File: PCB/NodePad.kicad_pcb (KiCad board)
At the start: 4 copper layers, 100 x 100 mm, 0 parts

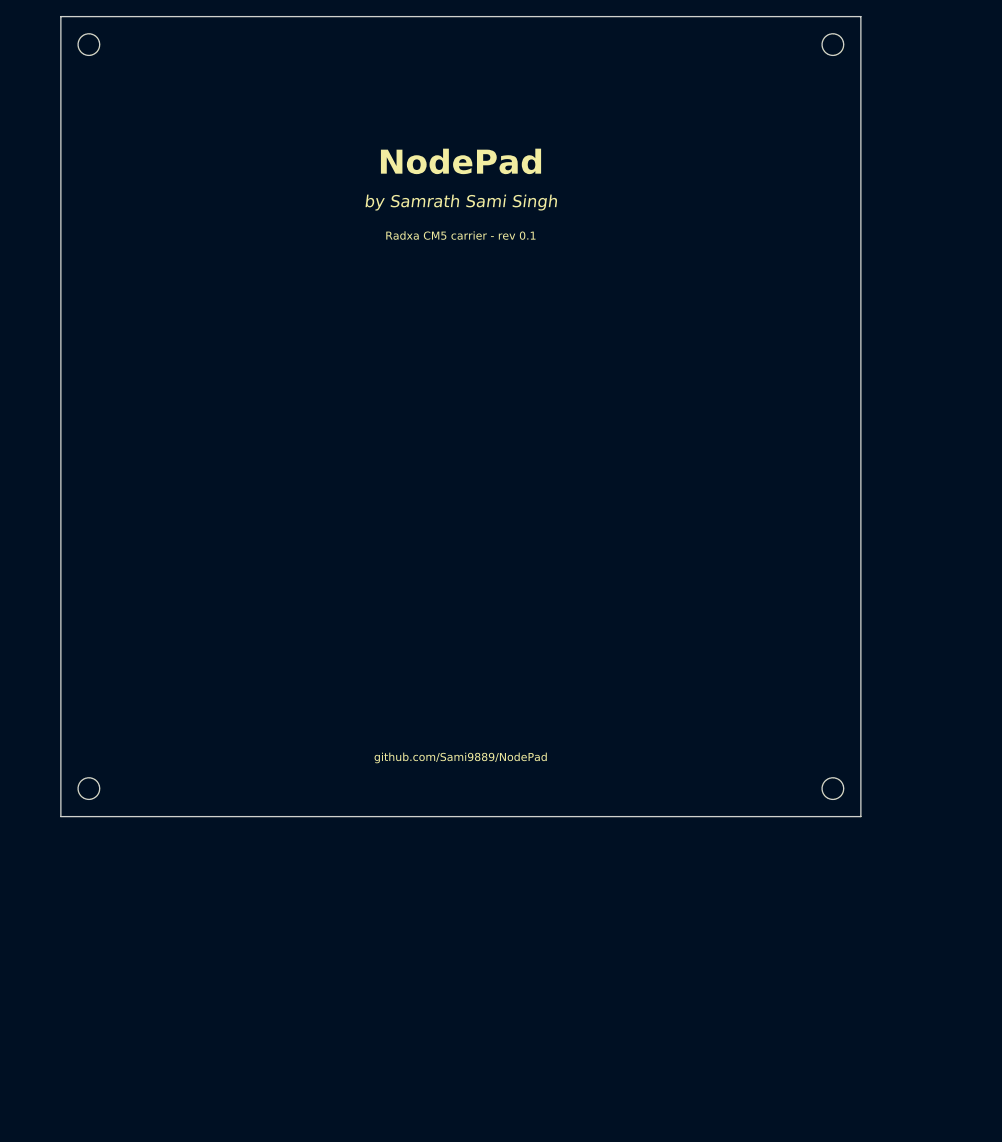
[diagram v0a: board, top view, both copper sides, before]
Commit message: Auto-generated changes
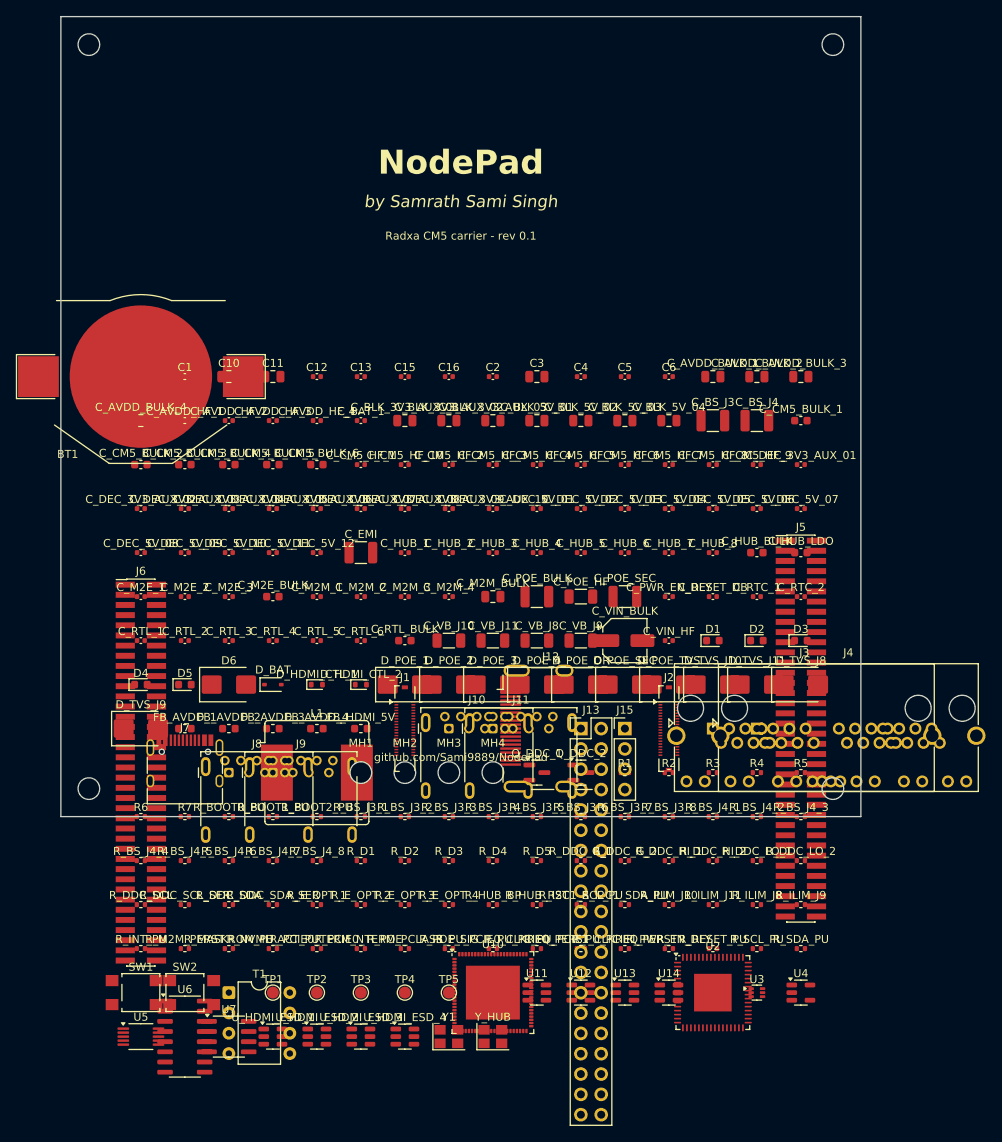
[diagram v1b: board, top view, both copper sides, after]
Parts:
- added BT1: CR2032, BatteryHolder_Keystone_3002_1x2032, F.Cu at (10.0, 45.0)
- added C1: 1uF, C_0402_1005Metric, F.Cu at (15.5, 45.0)
- added C10: 22uF/25V, C_0805_2012Metric, F.Cu at (21.0, 45.0)
- added C11: 22uF/25V, C_0805_2012Metric, F.Cu at (26.5, 45.0)
- added C12: 10uF/16V, C_0402_1005Metric, F.Cu at (32.0, 45.0)
- added C13: 100nF, C_0402_1005Metric, F.Cu at (37.5, 45.0)
- added C15: 1uF, C_0402_1005Metric, F.Cu at (43.0, 45.0)
- added C16: 1uF, C_0402_1005Metric, F.Cu at (48.5, 45.0)
- added C2: 1uF, C_0402_1005Metric, F.Cu at (54.0, 45.0)
- added C3: 22uF/25V, C_0805_2012Metric, F.Cu at (59.5, 45.0)
- added C4: 100nF, C_0402_1005Metric, F.Cu at (65.0, 45.0)
- added C5: 2.2nF, C_0402_1005Metric, F.Cu at (70.5, 45.0)
- added C6: 100pF, C_0402_1005Metric, F.Cu at (76.0, 45.0)
- added C_AVDD_BULK_1: 10uF, C_0805_2012Metric, F.Cu at (81.5, 45.0)
- added C_AVDD_BULK_2: 10uF, C_0805_2012Metric, F.Cu at (87.0, 45.0)
- added C_AVDD_BULK_3: 10uF, C_0805_2012Metric, F.Cu at (92.5, 45.0)
- added C_AVDD_BULK_4: 10uF, C_0805_2012Metric, F.Cu at (10.0, 50.5)
- added C_AVDD_HF_1: 100nF, C_0402_1005Metric, F.Cu at (15.5, 50.5)
- added C_AVDD_HF_2: 100nF, C_0402_1005Metric, F.Cu at (21.0, 50.5)
- added C_AVDD_HF_3: 100nF, C_0402_1005Metric, F.Cu at (26.5, 50.5)
- added C_AVDD_HF_4: 100nF, C_0402_1005Metric, F.Cu at (32.0, 50.5)
- added C_BAT_1: 100nF, C_0402_1005Metric, F.Cu at (37.5, 50.5)
- added C_BLK_3V3_AUX_01: 10uF, C_0805_2012Metric, F.Cu at (43.0, 50.5)
- added C_BLK_3V3_AUX_02: 10uF, C_0805_2012Metric, F.Cu at (48.5, 50.5)
- added C_BLK_3V3_AUX_03: 10uF, C_0805_2012Metric, F.Cu at (54.0, 50.5)
- added C_BLK_5V_01: 10uF, C_0805_2012Metric, F.Cu at (59.5, 50.5)
- added C_BLK_5V_02: 10uF, C_0805_2012Metric, F.Cu at (65.0, 50.5)
- added C_BLK_5V_03: 10uF, C_0805_2012Metric, F.Cu at (70.5, 50.5)
- added C_BLK_5V_04: 10uF, C_0805_2012Metric, F.Cu at (76.0, 50.5)
- added C_BS_J3: 1nF/2kV, C_1210_3225Metric, F.Cu at (81.5, 50.5)
- added C_BS_J4: 1nF/2kV, C_1210_3225Metric, F.Cu at (87.0, 50.5)
- added C_CM5_BULK_1: 10uF, C_0603_1608Metric, F.Cu at (92.5, 50.5)
- added C_CM5_BULK_2: 10uF, C_0603_1608Metric, F.Cu at (10.0, 56.0)
- added C_CM5_BULK_3: 10uF, C_0603_1608Metric, F.Cu at (15.5, 56.0)
- added C_CM5_BULK_4: 10uF, C_0603_1608Metric, F.Cu at (21.0, 56.0)
- added C_CM5_BULK_5: 10uF, C_0603_1608Metric, F.Cu at (26.5, 56.0)
- added C_CM5_BULK_6: 10uF, C_0603_1608Metric, F.Cu at (32.0, 56.0)
- added C_CM5_HF_1: 100nF, C_0402_1005Metric, F.Cu at (37.5, 56.0)
- added C_CM5_HF_10: 100nF, C_0402_1005Metric, F.Cu at (43.0, 56.0)
- added C_CM5_HF_2: 100nF, C_0402_1005Metric, F.Cu at (48.5, 56.0)
- added C_CM5_HF_3: 100nF, C_0402_1005Metric, F.Cu at (54.0, 56.0)
- added C_CM5_HF_4: 100nF, C_0402_1005Metric, F.Cu at (59.5, 56.0)
- added C_CM5_HF_5: 100nF, C_0402_1005Metric, F.Cu at (65.0, 56.0)
- added C_CM5_HF_6: 100nF, C_0402_1005Metric, F.Cu at (70.5, 56.0)
- added C_CM5_HF_7: 100nF, C_0402_1005Metric, F.Cu at (76.0, 56.0)
- added C_CM5_HF_8: 100nF, C_0402_1005Metric, F.Cu at (81.5, 56.0)
- added C_CM5_HF_9: 100nF, C_0402_1005Metric, F.Cu at (87.0, 56.0)
- added C_DEC_3V3_AUX_01: 100nF, C_0402_1005Metric, F.Cu at (92.5, 56.0)
- added C_DEC_3V3_AUX_02: 100nF, C_0402_1005Metric, F.Cu at (10.0, 61.5)
- added C_DEC_3V3_AUX_03: 100nF, C_0402_1005Metric, F.Cu at (15.5, 61.5)
- added C_DEC_3V3_AUX_04: 100nF, C_0402_1005Metric, F.Cu at (21.0, 61.5)
- added C_DEC_3V3_AUX_05: 100nF, C_0402_1005Metric, F.Cu at (26.5, 61.5)
- added C_DEC_3V3_AUX_06: 100nF, C_0402_1005Metric, F.Cu at (32.0, 61.5)
- added C_DEC_3V3_AUX_07: 100nF, C_0402_1005Metric, F.Cu at (37.5, 61.5)
- added C_DEC_3V3_AUX_08: 100nF, C_0402_1005Metric, F.Cu at (43.0, 61.5)
- added C_DEC_3V3_AUX_09: 100nF, C_0402_1005Metric, F.Cu at (48.5, 61.5)
- added C_DEC_3V3_AUX_10: 100nF, C_0402_1005Metric, F.Cu at (54.0, 61.5)
- added C_DEC_5V_01: 100nF, C_0402_1005Metric, F.Cu at (59.5, 61.5)
- added C_DEC_5V_02: 100nF, C_0402_1005Metric, F.Cu at (65.0, 61.5)
- added C_DEC_5V_03: 100nF, C_0402_1005Metric, F.Cu at (70.5, 61.5)
- added C_DEC_5V_04: 100nF, C_0402_1005Metric, F.Cu at (76.0, 61.5)
- added C_DEC_5V_05: 100nF, C_0402_1005Metric, F.Cu at (81.5, 61.5)
- added C_DEC_5V_06: 100nF, C_0402_1005Metric, F.Cu at (87.0, 61.5)
- added C_DEC_5V_07: 100nF, C_0402_1005Metric, F.Cu at (92.5, 61.5)
- added C_DEC_5V_08: 100nF, C_0402_1005Metric, F.Cu at (10.0, 67.0)
- added C_DEC_5V_09: 100nF, C_0402_1005Metric, F.Cu at (15.5, 67.0)
- added C_DEC_5V_10: 100nF, C_0402_1005Metric, F.Cu at (21.0, 67.0)
- added C_DEC_5V_11: 100nF, C_0402_1005Metric, F.Cu at (26.5, 67.0)
- added C_DEC_5V_12: 100nF, C_0402_1005Metric, F.Cu at (32.0, 67.0)
- added C_EMI: 1nF/2kV, C_1210_3225Metric, F.Cu at (37.5, 67.0)
- added C_HUB_1: 100nF, C_0402_1005Metric, F.Cu at (43.0, 67.0)
- added C_HUB_2: 100nF, C_0402_1005Metric, F.Cu at (48.5, 67.0)
- added C_HUB_3: 100nF, C_0402_1005Metric, F.Cu at (54.0, 67.0)
- added C_HUB_4: 100nF, C_0402_1005Metric, F.Cu at (59.5, 67.0)
- added C_HUB_5: 100nF, C_0402_1005Metric, F.Cu at (65.0, 67.0)
- added C_HUB_6: 100nF, C_0402_1005Metric, F.Cu at (70.5, 67.0)
- added C_HUB_7: 100nF, C_0402_1005Metric, F.Cu at (76.0, 67.0)
- added C_HUB_8: 100nF, C_0402_1005Metric, F.Cu at (81.5, 67.0)
- added C_HUB_BULK: 10uF, C_0603_1608Metric, F.Cu at (87.0, 67.0)
- added C_HUB_LDO: 4.7uF, C_0603_1608Metric, F.Cu at (92.5, 67.0)
- added C_M2E_1: 100nF, C_0402_1005Metric, F.Cu at (10.0, 72.5)
- added C_M2E_2: 100nF, C_0402_1005Metric, F.Cu at (15.5, 72.5)
- added C_M2E_3: 100nF, C_0402_1005Metric, F.Cu at (21.0, 72.5)
- added C_M2E_BULK: 10uF, C_0603_1608Metric, F.Cu at (26.5, 72.5)
- added C_M2M_1: 100nF, C_0402_1005Metric, F.Cu at (32.0, 72.5)
- added C_M2M_2: 100nF, C_0402_1005Metric, F.Cu at (37.5, 72.5)
- added C_M2M_3: 100nF, C_0402_1005Metric, F.Cu at (43.0, 72.5)
- added C_M2M_4: 100nF, C_0402_1005Metric, F.Cu at (48.5, 72.5)
- added C_M2M_BULK: 22uF/6.3V, C_0805_2012Metric, F.Cu at (54.0, 72.5)
- added C_POE_BULK: 22uF/100V DNP, C_1210_3225Metric, F.Cu at (59.5, 72.5)
- added C_POE_HF: 100nF/100V DNP, C_1206_3216Metric, F.Cu at (65.0, 72.5)
- added C_POE_SEC: 47uF/25V DNP, C_1210_3225Metric, F.Cu at (70.5, 72.5)
- added C_PWR_EN_DLY: 470nF, C_0402_1005Metric, F.Cu at (76.0, 72.5)
- added C_RESET_DB: 100nF, C_0402_1005Metric, F.Cu at (81.5, 72.5)
- added C_RTC_1: 100nF, C_0402_1005Metric, F.Cu at (87.0, 72.5)
- added C_RTC_2: 1uF, C_0402_1005Metric, F.Cu at (92.5, 72.5)
- added C_RTL_1: 100nF, C_0402_1005Metric, F.Cu at (10.0, 78.0)
- added C_RTL_2: 100nF, C_0402_1005Metric, F.Cu at (15.5, 78.0)
- added C_RTL_3: 100nF, C_0402_1005Metric, F.Cu at (21.0, 78.0)
- added C_RTL_4: 100nF, C_0402_1005Metric, F.Cu at (26.5, 78.0)
- added C_RTL_5: 100nF, C_0402_1005Metric, F.Cu at (32.0, 78.0)
- added C_RTL_6: 100nF, C_0402_1005Metric, F.Cu at (37.5, 78.0)
- added C_RTL_BULK: 10uF, C_0603_1608Metric, F.Cu at (43.0, 78.0)
- added C_VB_J10: 150uF/6.3V, C_1206_3216Metric, F.Cu at (48.5, 78.0)
- added C_VB_J11: 150uF/6.3V, C_1206_3216Metric, F.Cu at (54.0, 78.0)
- added C_VB_J8: 150uF/6.3V, C_1206_3216Metric, F.Cu at (59.5, 78.0)
- added C_VB_J9: 150uF/6.3V, C_1206_3216Metric, F.Cu at (65.0, 78.0)
- added C_VIN_BULK: 47uF/25V, CP_Elec_5x5.4, F.Cu at (70.5, 78.0)
- added C_VIN_HF: 100nF, C_0402_1005Metric, F.Cu at (76.0, 78.0)
- added D1: Green, LED_0603_1608Metric, F.Cu at (81.5, 78.0)
- added D2: Blue, LED_0603_1608Metric, F.Cu at (87.0, 78.0)
- added D3: Yellow, LED_0603_1608Metric, F.Cu at (92.5, 78.0)
- added D4: Yellow, LED_0603_1608Metric, F.Cu at (10.0, 83.5)
- added D5: Red, LED_0603_1608Metric, F.Cu at (15.5, 83.5)
- added D6: SMBJ12A, D_SMB, F.Cu at (21.0, 83.5)
- added D_BAT: BAT54, D_SOD-323, F.Cu at (26.5, 83.5)
- added D_HDMI_CTL_1: ESD5Z5.0, D_SOD-523, F.Cu at (32.0, 83.5)
- added D_HDMI_CTL_2: ESD5Z5.0, D_SOD-523, F.Cu at (37.5, 83.5)
- added D_POE_1: HD01-T DNP, D_SMB, F.Cu at (43.0, 83.5)
- added D_POE_2: HD01-T DNP, D_SMB, F.Cu at (48.5, 83.5)
- added D_POE_3: HD01-T DNP, D_SMB, F.Cu at (54.0, 83.5)
- added D_POE_4: HD01-T DNP, D_SMB, F.Cu at (59.5, 83.5)
- added D_POE_OR: SS36 DNP, D_SMB, F.Cu at (65.0, 83.5)
- added D_POE_SEC: SS36 DNP, D_SMB, F.Cu at (70.5, 83.5)
- added D_POE_TVS: SMBJ58A DNP, D_SMB, F.Cu at (76.0, 83.5)
- added D_TVS_J10: SMBJ5.0A, D_SMB, F.Cu at (81.5, 83.5)
- added D_TVS_J11: SMBJ5.0A, D_SMB, F.Cu at (87.0, 83.5)
- added D_TVS_J8: SMBJ5.0A, D_SMB, F.Cu at (92.5, 83.5)
- added D_TVS_J9: SMBJ5.0A, D_SMB, F.Cu at (10.0, 89.0)
- added FB_AVDD_1: 600R@100MHz, L_0603_1608Metric, F.Cu at (15.5, 89.0)
- added FB_AVDD_2: 600R@100MHz, L_0603_1608Metric, F.Cu at (21.0, 89.0)
- added FB_AVDD_3: 600R@100MHz, L_0603_1608Metric, F.Cu at (26.5, 89.0)
- added FB_AVDD_4: 600R@100MHz, L_0603_1608Metric, F.Cu at (32.0, 89.0)
- added FB_HDMI_5V: 600R@100MHz, L_0603_1608Metric, F.Cu at (37.5, 89.0)
- added J1: CM5-J1, Hirose_BM24_BM24-40DS-2-0.35V_2x20_P0.35mm_PowerPin2_Vertical, F.Cu at (43.0, 89.0)
- added J10: USB3-A, USB3_A_Molex_48393-001, F.Cu at (48.5, 89.0)
- added J11: USB3-A, USB3_A_Molex_48393-001, F.Cu at (54.0, 89.0)
- added J12: HDMI, HDMI_A_Molex_208658-1001_Horizontal, F.Cu at (59.5, 89.0)
- added J13: GPIO40, PinHeader_2x20_P2.54mm_Vertical, F.Cu at (65.0, 89.0)
- added J15: Fan, PinHeader_1x04_P2.54mm_Vertical, F.Cu at (70.5, 89.0)
- added J2: CM5-J2, Hirose_BM24_BM24-40DS-2-0.35V_2x20_P0.35mm_PowerPin2_Vertical, F.Cu at (76.0, 89.0)
- added J3: RJ45, RJ45_Amphenol_RJHSE538X-02, F.Cu at (81.5, 89.0)
- added J4: RJ45, RJ45_Amphenol_RJHSE538X-02, F.Cu at (87.0, 89.0)
- added J5: M.2 M-key 2280, PinHeader_2x38_P1.27mm_Vertical_SMD, F.Cu at (92.5, 89.0)
- added J6: M.2 E-key 2230, PinHeader_2x38_P1.27mm_Vertical_SMD, F.Cu at (10.0, 94.5)
- added J7: USB-C, USB_C_Receptacle_HRO_TYPE-C-31-M-12, F.Cu at (15.5, 94.5)
- added J8: USB3-A, USB3_A_Molex_48393-001, F.Cu at (21.0, 94.5)
- added J9: USB3-A, USB3_A_Molex_48393-001, F.Cu at (26.5, 94.5)
- added L1: 4.7uH/3A, L_Bourns_SRR1208_12.7x12.7mm, F.Cu at (32.0, 94.5)
- added MH1: M2.5 heatsink, MountingHole_2.7mm_M2.5, F.Cu at (37.5, 94.5)
- added MH2: M2.5 heatsink, MountingHole_2.7mm_M2.5, F.Cu at (43.0, 94.5)
- added MH3: M2.5 heatsink, MountingHole_2.7mm_M2.5, F.Cu at (48.5, 94.5)
- added MH4: M2.5 heatsink, MountingHole_2.7mm_M2.5, F.Cu at (54.0, 94.5)
- added Q_DDC_1: BSS138, SOT-23, F.Cu at (59.5, 94.5)
- added Q_DDC_2: BSS138, SOT-23, F.Cu at (65.0, 94.5)
- added R1: 10k, R_0402_1005Metric, F.Cu at (70.5, 94.5)
- added R2: 10k, R_0402_1005Metric, F.Cu at (76.0, 94.5)
- added R3: 0, R_0402_1005Metric, F.Cu at (81.5, 94.5)
- added R4: 100k, R_0402_1005Metric, F.Cu at (87.0, 94.5)
- added R5: 52.3k, R_0402_1005Metric, F.Cu at (92.5, 94.5)
- added R6: 10k, R_0402_1005Metric, F.Cu at (10.0, 100.0)
- added R7: 10k, R_0402_1005Metric, F.Cu at (15.5, 100.0)
- added R_BOOT0_PU: 10k, R_0402_1005Metric, F.Cu at (21.0, 100.0)
- added R_BOOT1_PU: 10k, R_0402_1005Metric, F.Cu at (26.5, 100.0)
- added R_BOOT2_PU: 10k, R_0402_1005Metric, F.Cu at (32.0, 100.0)
- added R_BS_J3_1: 75, R_0402_1005Metric, F.Cu at (37.5, 100.0)
- added R_BS_J3_2: 75, R_0402_1005Metric, F.Cu at (43.0, 100.0)
- added R_BS_J3_3: 75, R_0402_1005Metric, F.Cu at (48.5, 100.0)
- added R_BS_J3_4: 75, R_0402_1005Metric, F.Cu at (54.0, 100.0)
- added R_BS_J3_5: 75, R_0402_1005Metric, F.Cu at (59.5, 100.0)
- added R_BS_J3_6: 75, R_0402_1005Metric, F.Cu at (65.0, 100.0)
- added R_BS_J3_7: 75, R_0402_1005Metric, F.Cu at (70.5, 100.0)
- added R_BS_J3_8: 75, R_0402_1005Metric, F.Cu at (76.0, 100.0)
- added R_BS_J4_1: 75, R_0402_1005Metric, F.Cu at (81.5, 100.0)
- added R_BS_J4_2: 75, R_0402_1005Metric, F.Cu at (87.0, 100.0)
- added R_BS_J4_3: 75, R_0402_1005Metric, F.Cu at (92.5, 100.0)
- added R_BS_J4_4: 75, R_0402_1005Metric, F.Cu at (10.0, 105.5)
- added R_BS_J4_5: 75, R_0402_1005Metric, F.Cu at (15.5, 105.5)
- added R_BS_J4_6: 75, R_0402_1005Metric, F.Cu at (21.0, 105.5)
- added R_BS_J4_7: 75, R_0402_1005Metric, F.Cu at (26.5, 105.5)
- added R_BS_J4_8: 75, R_0402_1005Metric, F.Cu at (32.0, 105.5)
- added R_D1: 1k, R_0402_1005Metric, F.Cu at (37.5, 105.5)
- added R_D2: 1k, R_0402_1005Metric, F.Cu at (43.0, 105.5)
- added R_D3: 1k, R_0402_1005Metric, F.Cu at (48.5, 105.5)
- added R_D4: 1k, R_0402_1005Metric, F.Cu at (54.0, 105.5)
- added R_D5: 1k, R_0402_1005Metric, F.Cu at (59.5, 105.5)
- added R_DDC_G_1: 10k, R_0402_1005Metric, F.Cu at (65.0, 105.5)
- added R_DDC_G_2: 10k, R_0402_1005Metric, F.Cu at (70.5, 105.5)
- added R_DDC_HI_1: 10k, R_0402_1005Metric, F.Cu at (76.0, 105.5)
- added R_DDC_HI_2: 10k, R_0402_1005Metric, F.Cu at (81.5, 105.5)
- added R_DDC_LO_1: 10k, R_0402_1005Metric, F.Cu at (87.0, 105.5)
- added R_DDC_LO_2: 10k, R_0402_1005Metric, F.Cu at (92.5, 105.5)
- added R_DDC_SCL: 2.2k, R_0402_1005Metric, F.Cu at (10.0, 111.0)
- added R_DDC_SCL_SER: 100, R_0402_1005Metric, F.Cu at (15.5, 111.0)
- added R_DDC_SDA: 2.2k, R_0402_1005Metric, F.Cu at (21.0, 111.0)
- added R_DDC_SDA_SER: 100, R_0402_1005Metric, F.Cu at (26.5, 111.0)
- added R_E_OPT_1: 0/DNP, R_0402_1005Metric, F.Cu at (32.0, 111.0)
- added R_E_OPT_2: 0/DNP, R_0402_1005Metric, F.Cu at (37.5, 111.0)
- added R_E_OPT_3: 0/DNP, R_0402_1005Metric, F.Cu at (43.0, 111.0)
- added R_E_OPT_4: 0/DNP, R_0402_1005Metric, F.Cu at (48.5, 111.0)
- added R_HUB_BP: 10k, R_0402_1005Metric, F.Cu at (54.0, 111.0)
- added R_HUB_RST: 10k, R_0402_1005Metric, F.Cu at (59.5, 111.0)
- added R_I2C1_SCL_PU: 4.7k, R_0402_1005Metric, F.Cu at (65.0, 111.0)
- added R_I2C1_SDA_PU: 4.7k, R_0402_1005Metric, F.Cu at (70.5, 111.0)
- added R_ILIM_J10: 30k, R_0402_1005Metric, F.Cu at (76.0, 111.0)
- added R_ILIM_J11: 30k, R_0402_1005Metric, F.Cu at (81.5, 111.0)
- added R_ILIM_J8: 30k, R_0402_1005Metric, F.Cu at (87.0, 111.0)
- added R_ILIM_J9: 30k, R_0402_1005Metric, F.Cu at (92.5, 111.0)
- added R_INT_PU: 10k, R_0402_1005Metric, F.Cu at (10.0, 116.5)
- added R_M2M_PERST: 10k, R_0402_1005Metric, F.Cu at (15.5, 116.5)
- added R_MASKROM_PU: 10k, R_0402_1005Metric, F.Cu at (21.0, 116.5)
- added R_NVME_ACT_PU: 10k, R_0402_1005Metric, F.Cu at (26.5, 116.5)
- added R_PCIE0_TERM_N: 49.9 DNP, R_0402_1005Metric, F.Cu at (32.0, 116.5)
- added R_PCIE0_TERM_P: 49.9 DNP, R_0402_1005Metric, F.Cu at (37.5, 116.5)
- added R_POE_CLASS: 12.5 DNP, R_0402_1005Metric, F.Cu at (43.0, 116.5)
- added R_POE_SIG: 25k DNP, R_0402_1005Metric, F.Cu at (48.5, 116.5)
- added R_PU_PCIE0_CLKREQ: 10k, R_0402_1005Metric, F.Cu at (54.0, 116.5)
- added R_PU_PCIE0_PERST: 10k, R_0402_1005Metric, F.Cu at (59.5, 116.5)
- added R_PU_PCIE1_CLKREQ: 10k, R_0402_1005Metric, F.Cu at (65.0, 116.5)
- added R_PU_PCIE1_PERST: 10k, R_0402_1005Metric, F.Cu at (70.5, 116.5)
- added R_PWR_EN_DLY: 100k, R_0402_1005Metric, F.Cu at (76.0, 116.5)
- added R_RESET_PU: 10k, R_0402_1005Metric, F.Cu at (81.5, 116.5)
- added R_SCL_PU: 4.7k, R_0402_1005Metric, F.Cu at (87.0, 116.5)
- added R_SDA_PU: 4.7k, R_0402_1005Metric, F.Cu at (92.5, 116.5)
- added SW1: RESET, SW_SPST_TL3305A, F.Cu at (10.0, 122.0)
- added SW2: BOOT, SW_SPST_TL3305A, F.Cu at (15.5, 122.0)
- added T1: 750317847 DNP, DIP-8_W7.62mm, F.Cu at (21.0, 122.0)
- added TP1: TP, TestPoint_Pad_D1.5mm, F.Cu at (26.5, 122.0)
- added TP2: TP, TestPoint_Pad_D1.5mm, F.Cu at (32.0, 122.0)
- added TP3: TP, TestPoint_Pad_D1.5mm, F.Cu at (37.5, 122.0)
- added TP4: TP, TestPoint_Pad_D1.5mm, F.Cu at (43.0, 122.0)
- added TP5: TP, TestPoint_Pad_D1.5mm, F.Cu at (48.5, 122.0)
- added U10: GL3523, ArtInChip_QFN-88-1EP_10x10mm_P0.4mm_EP6.74x6.74mm, F.Cu at (54.0, 122.0)
- added U11: TPS2553, SOT-23-6, F.Cu at (59.5, 122.0)
- added U12: TPS2553, SOT-23-6, F.Cu at (65.0, 122.0)
- added U13: TPS2553, SOT-23-6, F.Cu at (70.5, 122.0)
- added U14: TPS2553, SOT-23-6, F.Cu at (76.0, 122.0)
- added U2: RTL8125BG, QFN-64-1EP_9x9mm_P0.5mm_EP4.7x4.7mm, F.Cu at (81.5, 122.0)
- added U3: MP2315, SOT-563, F.Cu at (87.0, 122.0)
- added U4: AP2112K-3.3, SOT-23-5, F.Cu at (92.5, 122.0)
- added U5: CH224K, VSSOP-10_3x3mm_P0.5mm, F.Cu at (10.0, 127.5)
- added U6: MP8007 DNP, SOIC-16_3.9x9.9mm_P1.27mm, F.Cu at (15.5, 127.5)
- added U7: DS3231MZ+, SOIC-8_3.9x4.9mm_P1.27mm, F.Cu at (21.0, 127.5)
- added U_HDMI_ESD_1: USBLC6-2SC6, SOT-23-6, F.Cu at (26.5, 127.5)
- added U_HDMI_ESD_2: USBLC6-2SC6, SOT-23-6, F.Cu at (32.0, 127.5)
- added U_HDMI_ESD_3: USBLC6-2SC6, SOT-23-6, F.Cu at (37.5, 127.5)
- added U_HDMI_ESD_4: USBLC6-2SC6, SOT-23-6, F.Cu at (43.0, 127.5)
- added Y1: 25MHz TCXO, Crystal_SMD_3225-4Pin_3.2x2.5mm, F.Cu at (48.5, 127.5)
- added Y_HUB: 25MHz, Crystal_SMD_3225-4Pin_3.2x2.5mm, F.Cu at (54.0, 127.5)
